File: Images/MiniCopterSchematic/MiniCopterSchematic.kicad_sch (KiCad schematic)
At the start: 28 parts, among them M1 Motor_DC_1, M2 Motor_DC_2, M3 Motor_DC_3, M4 Motor_DC_4, Q1 FQP20NO6L, Q2 FQP20NO6L, Q3 FQP20NO6L, Q4 FQP20NO6L, U1 ARDUINO NANO, U2 MPU6050, U3 NRF24L01_Breakout

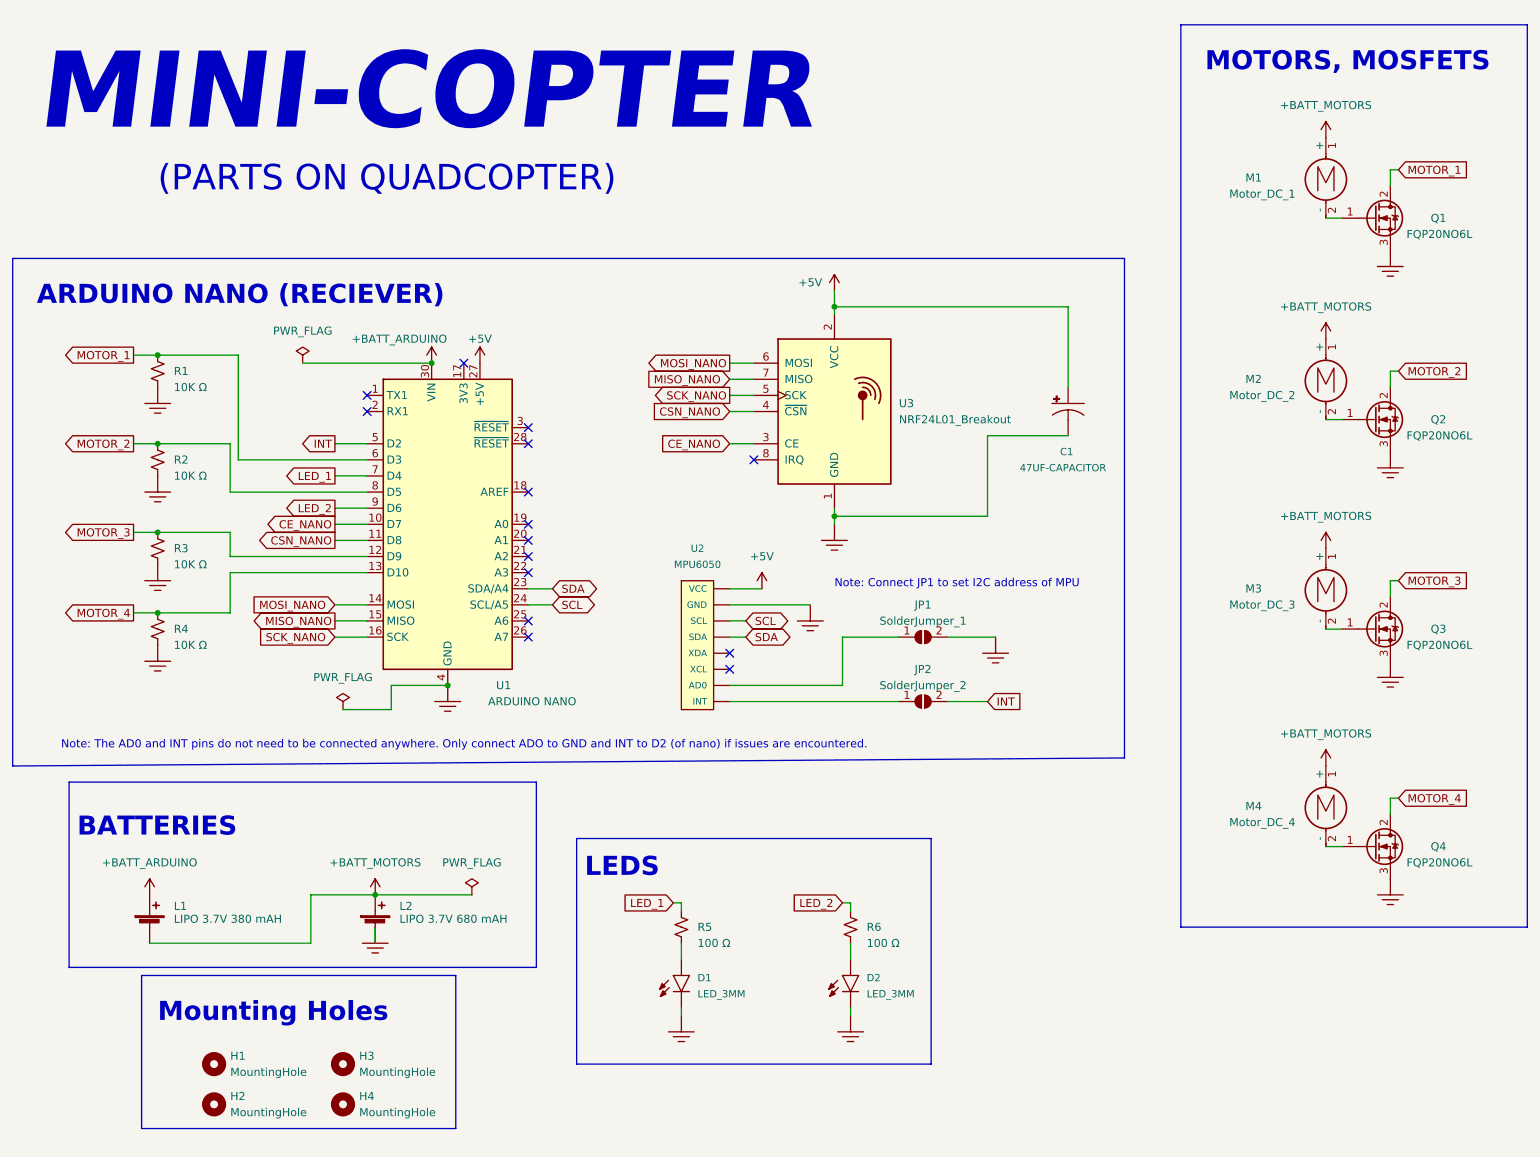
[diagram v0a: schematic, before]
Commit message: PCB design finalizing
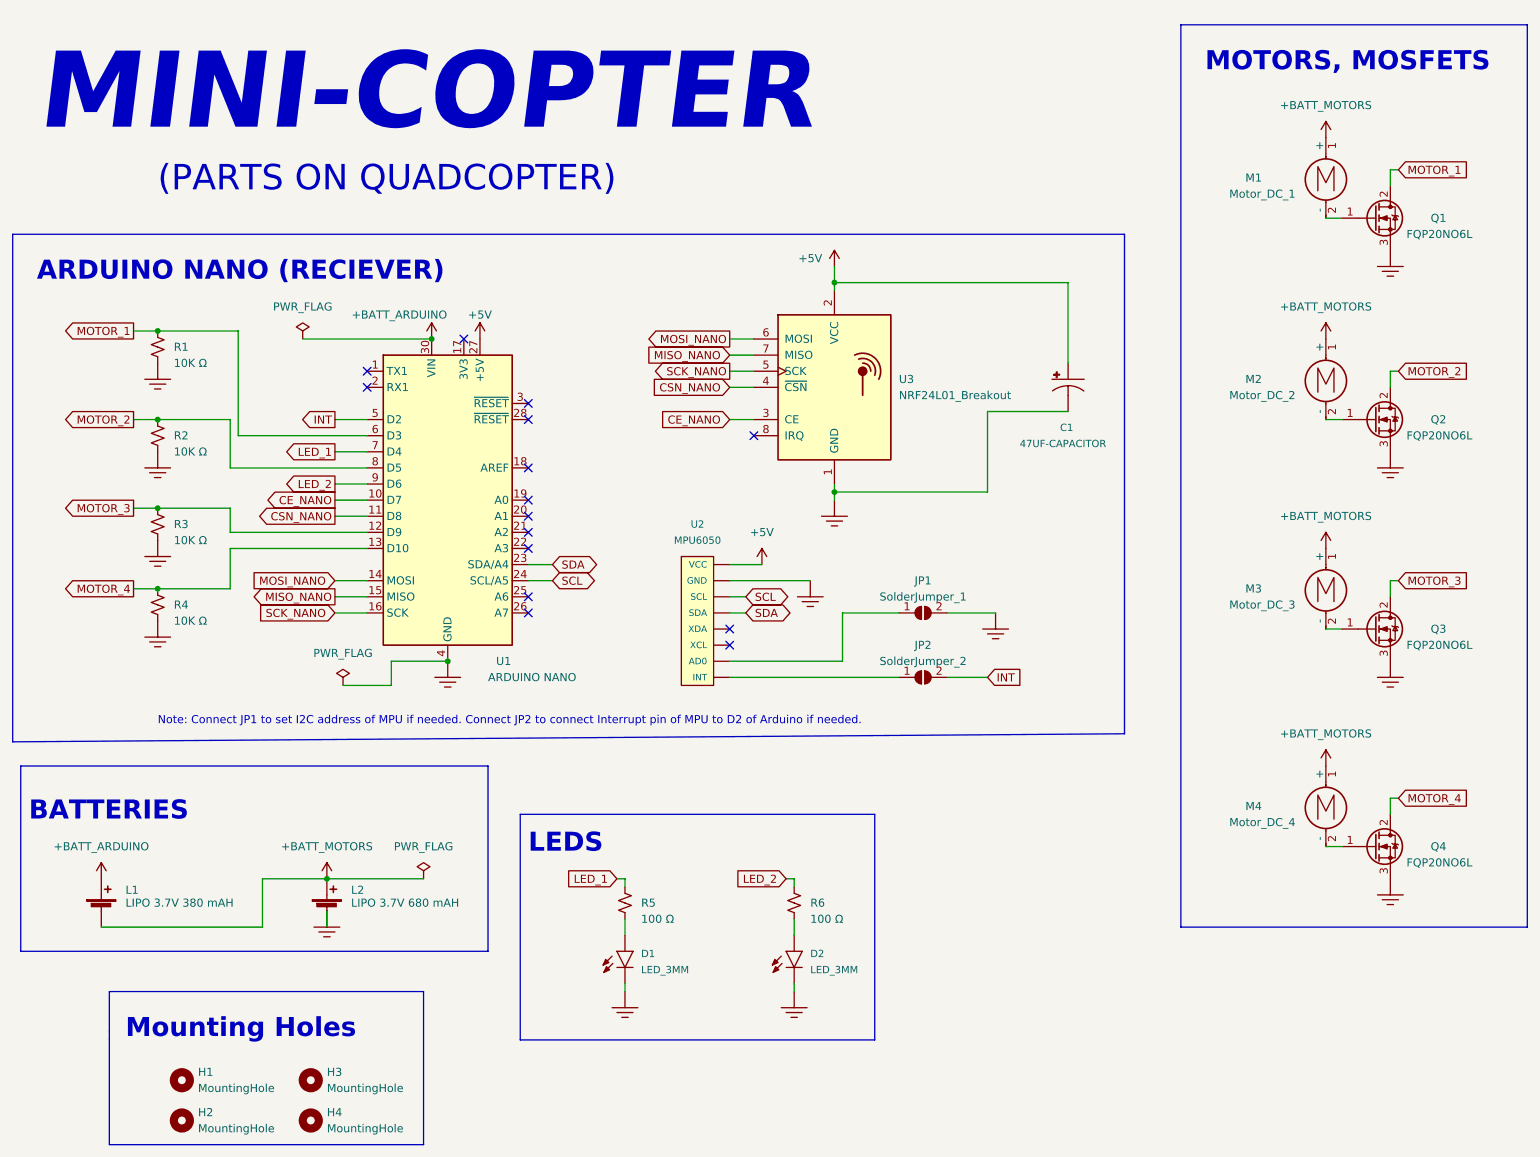
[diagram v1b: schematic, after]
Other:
- note added: "Note: Connect JP1 to set I2C address of MPU if needed. Connect JP2 to connect Interrupt pin of MPU to D2 of Arduino if needed."
- note removed: "Note: Connect JP1 to set I2C address of MPU"
- note removed: "Note: The AD0 and INT pins do not need to be connected anywhere. Only connect ADO to GND and INT to D2 (of nano) if issues are encountered."
- moved on the sheet: C1, D1, D2, H1, H2, H3, H4, JP1, JP2, L1, L2, R1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
